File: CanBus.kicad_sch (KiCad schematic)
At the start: 23 parts, among them J5 CAN INPUT, U1 STM32F446VETx, U2 SN65HVD230DR

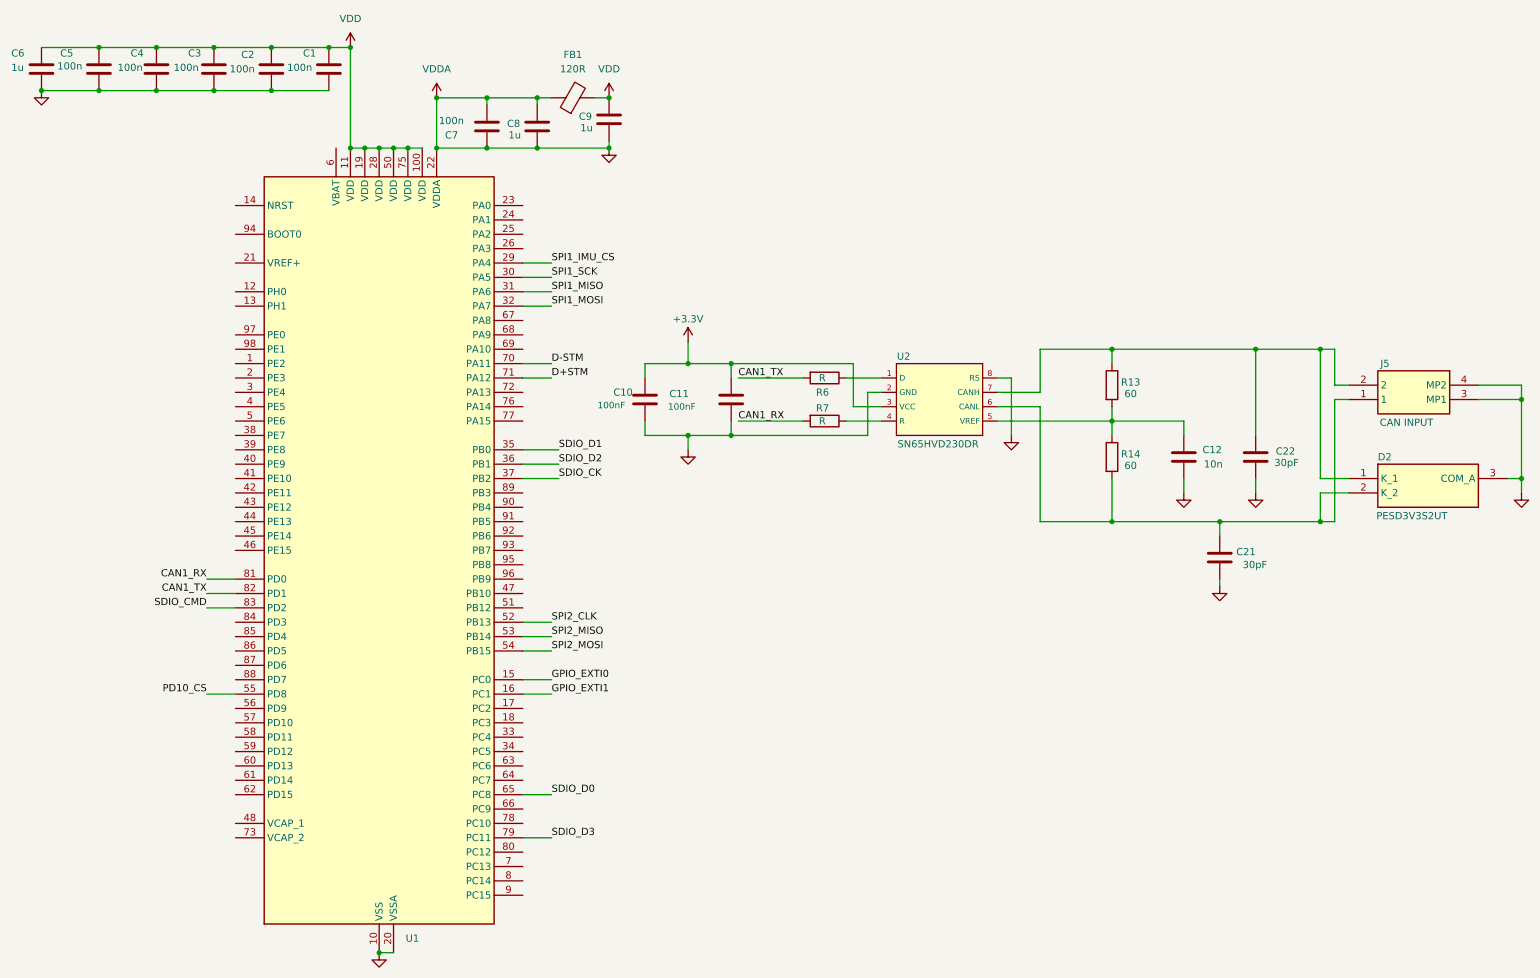
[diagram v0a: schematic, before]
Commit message: Feat: Added Canbus
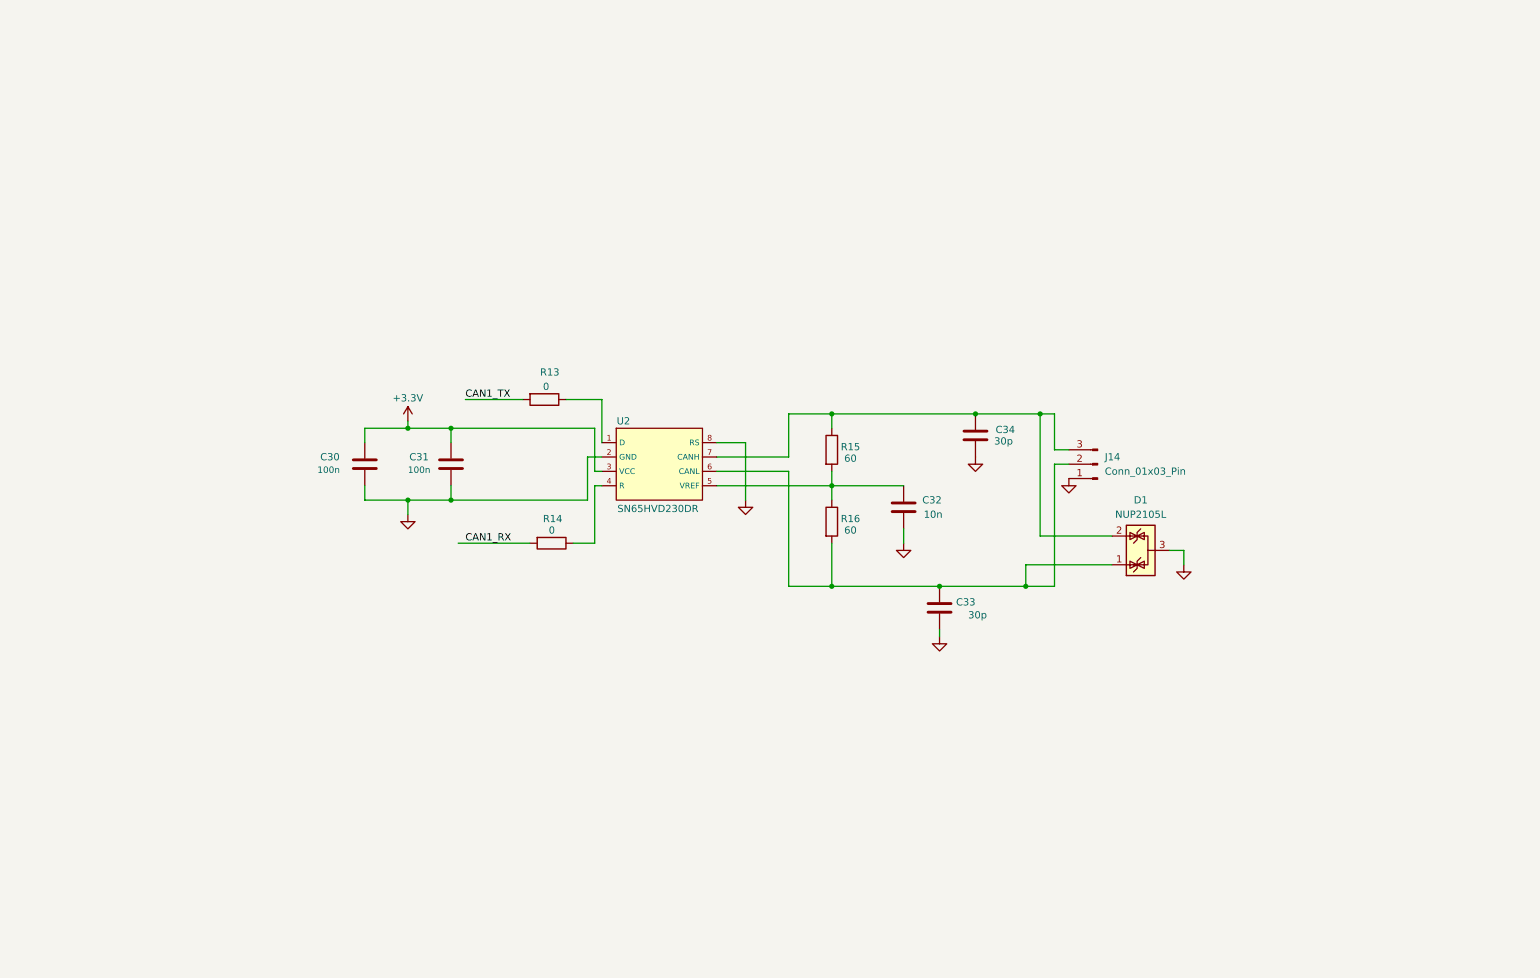
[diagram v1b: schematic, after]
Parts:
- removed C1, C2, C3, C4, C5, C7: 100n, symbol Device:C
- removed C10, C11: 100nF, symbol Device:C
- removed C12: 10n, symbol Device:C
- removed C21, C22: 30pF, symbol Device:C
- removed C6, C8, C9: 1u, symbol Device:C
- removed D2: PESD3V3S2UT, SOT95P230X110-3N, symbol SamacSys_Parts:PESD3V3S2UT
- removed FB1: 120R, symbol Device:FerriteBead
- removed J5: CAN INPUT, B2BPHSM4TBTLFSN, symbol SamacSys_Parts:B2B-PH-SM4-TBT_LF__SN_
- removed R6, R7: R, symbol Device:R
- removed U1: STM32F446VETx, Package_QFP:LQFP-100_14x14mm_P0.5mm, symbol MCU_ST_STM32F4:STM32F446VETx
- added C30, C31: 100n, symbol Device:C
- added C32: 10n, symbol Device:C
- added C33, C34: 30p, symbol Device:C
- added D1: NUP2105L, Package_TO_SOT_SMD:SOT-23, symbol Power_Protection:NUP2105L
- added J14: Conn_01x03_Pin, symbol Connector:Conn_01x03_Pin
- added R15, R16: 60, symbol Device:R
- R13, R14: value 60 -> 0
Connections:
- net +3.3V: now also C30.1, C31.1
- net CAN1_RX: now also R14.2
- net CAN1_TX: now also R13.2
- net GND: now also C30.2, C31.2, C32.2, C33.1, C34.1, D1.3 (A), J14.1 (Pin_1)
- net at U2.4 (R): now also R14.1
- net at U2.1 (D): now also R13.1
- net at U2.6 (CANL): now also C33.2, D1.1 (K), J14.2 (Pin_2), R16.2; no longer R14.2
- net at U2.7 (CANH): now also C34.2, D1.2 (K), J14.3 (Pin_3), R15.1; no longer R13.1
- new net: C32.1, R15.2, R16.1, U2.5 (VREF)
